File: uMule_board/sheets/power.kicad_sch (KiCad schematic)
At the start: 52 parts, among them Q1 AON6407, U1 TPS62933, U14 TPS62933, U2 TLV761, U3 INA219AxD

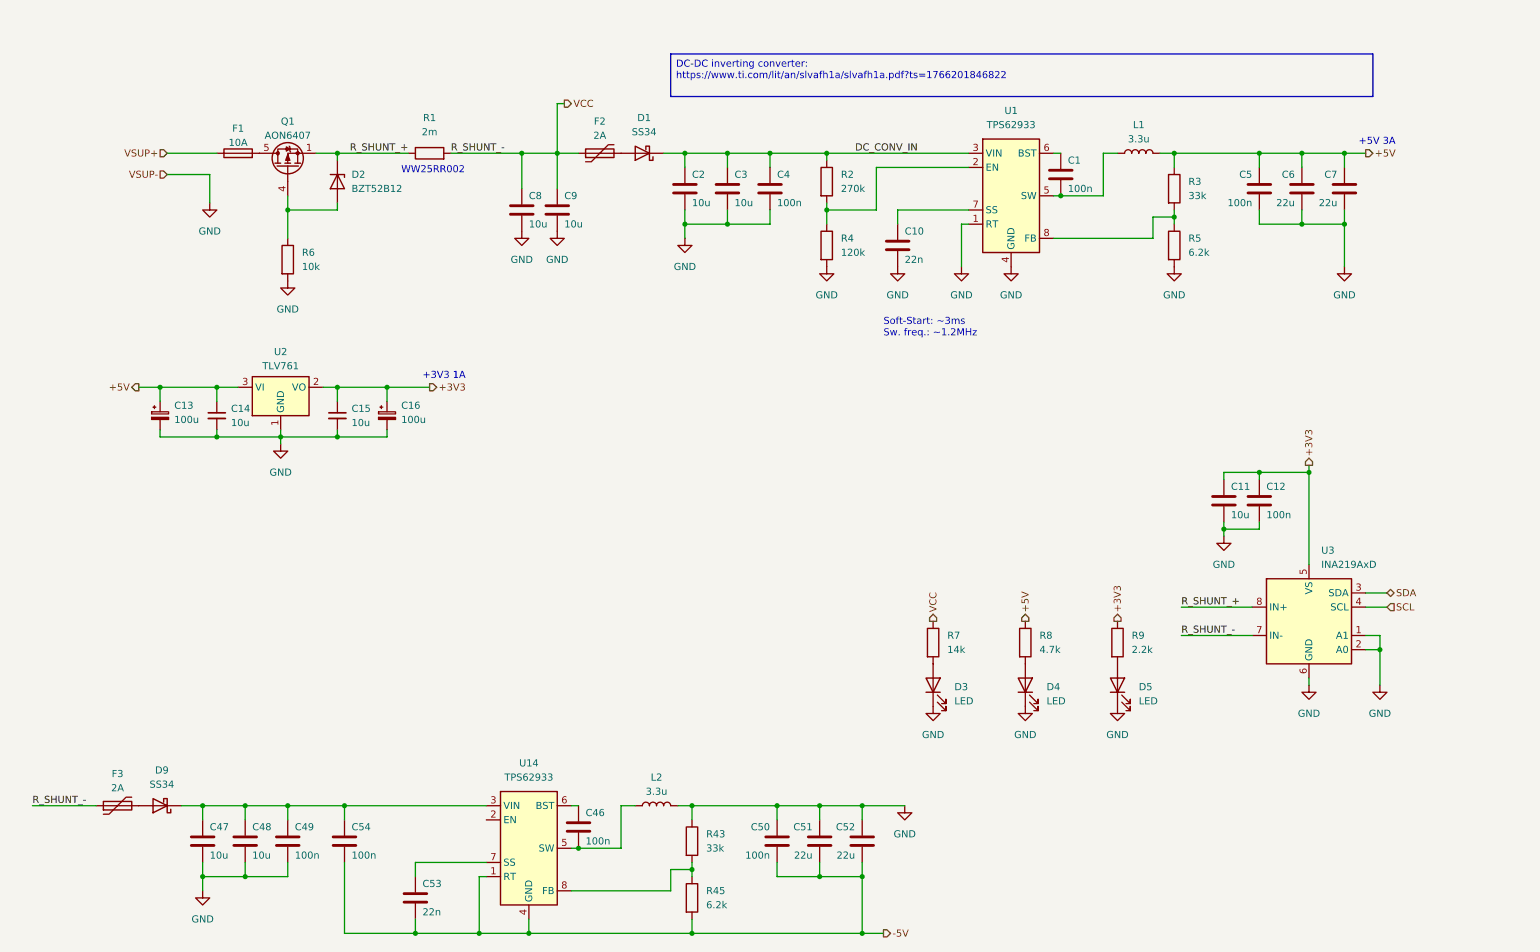
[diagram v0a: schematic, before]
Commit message: sch ready, only missing the pcb
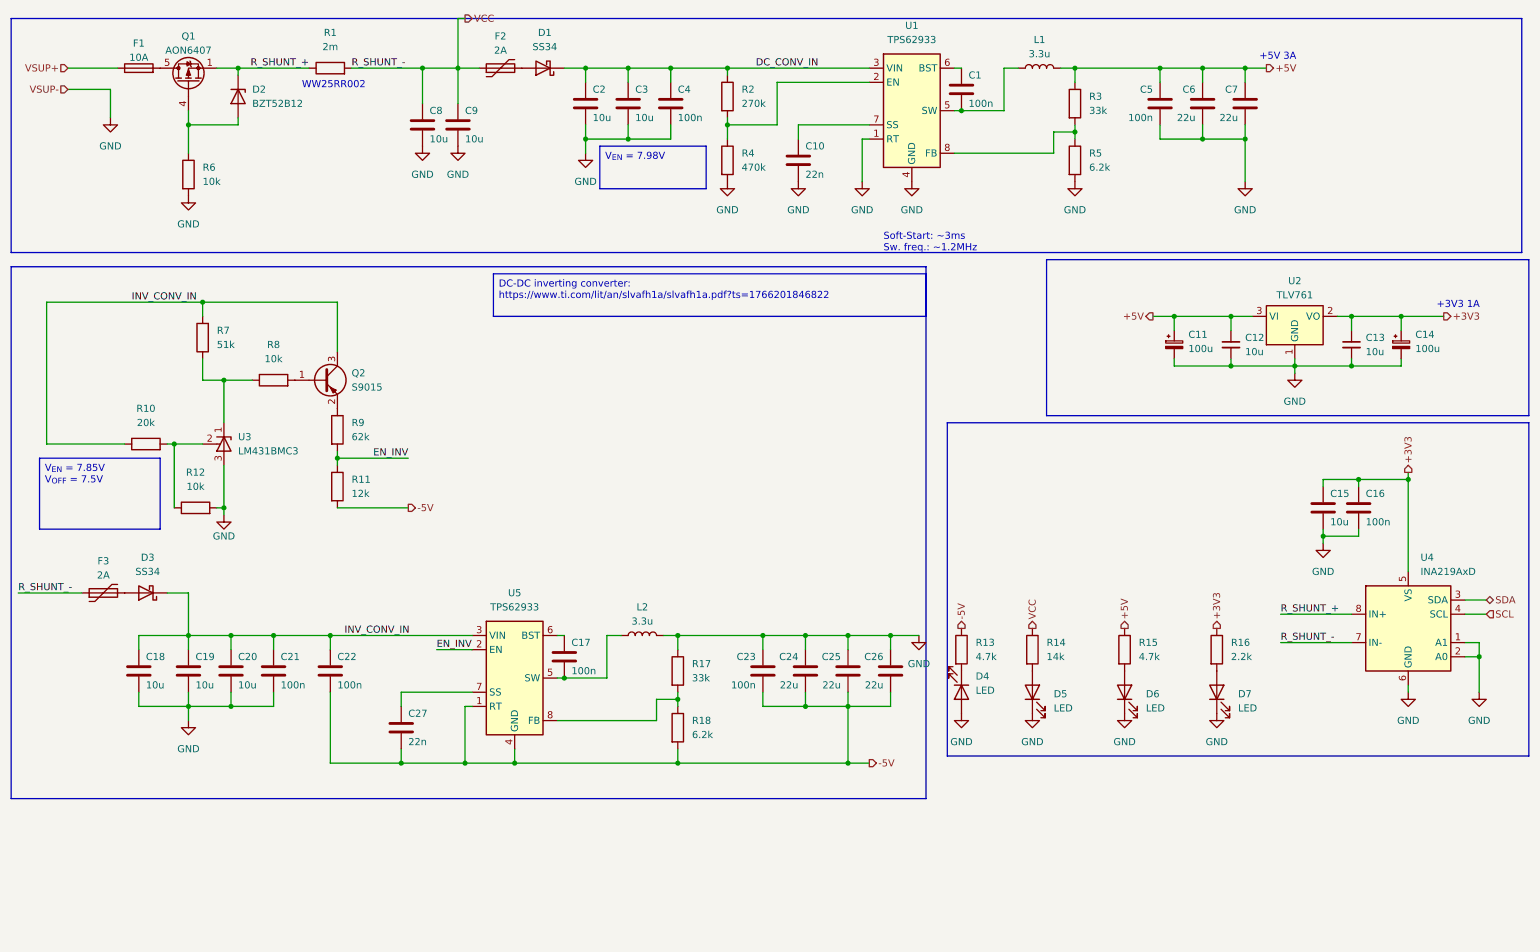
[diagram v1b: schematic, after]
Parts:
- added C18: 10u, Capacitor_SMD:C_0805_2012Metric, symbol Device:C
- added C26: 22u, Capacitor_SMD:C_0805_2012Metric, symbol Device:C
- added D4: LED, LED_SMD:LED_0603_1608Metric_Pad1.05x0.95mm_HandSolder, symbol Device:LED
- added Q2: S9015, Package_TO_SOT_SMD:SOT-23, symbol My_elemets:S9015
- added R10: 20k, Resistor_SMD:R_0603_1608Metric, symbol Device:R
- added R11: 12k, Resistor_SMD:R_0603_1608Metric, symbol Device:R
- added R12, R8: 10k, Resistor_SMD:R_0603_1608Metric, symbol Device:R
- added R13: 4.7k, Resistor_SMD:R_0603_1608Metric, symbol Device:R
- added R7: 51k, Resistor_SMD:R_0603_1608Metric, symbol Device:R
- added R9: 62k, Resistor_SMD:R_0603_1608Metric, symbol Device:R
- added U3: LM431BMC3, Package_TO_SOT_SMD:SOT-23, symbol My_elemets:LM431BMC3
- R4: value 120k -> 470k
- renumbered C13 to C11, C14 to C12, C15 to C13, C16 to C14, C11 to C15, C12 to C16, C46 to C17, C47 to C19, C48 to C20, C49 to C21, C54 to C22, C50 to C23, C51 to C24, C52 to C25, C53 to C27, D9 to D3, D3 to D5, D4 to D6, D5 to D7, R7 to R14, R8 to R15, R9 to R16, R43 to R17, R45 to R18, U3 to U4, U14 to U5
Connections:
- net -5V: now also C26.2, R11.2, R13.1
- net GND: now also C18.2, C26.1, D4.2 (A), R12.2, U3.3 (A)
- net INV_CONV_IN: now reaches C19.1, C20.1, C21.1, C22.1, D3.1 (K), U5.3 (VIN)
- net INV_CONV_IN: now also C18.1, Q2.3 (C), R10.1, R7.2
- net EN_INV: now reaches U5.2 (EN)
- net EN_INV: now also R11.1, R9.2
- new net: R10.2, R12.1, U3.2 (REF)
- new net: R7.1, R8.1, U3.1 (K)
- new net: Q2.1 (B), R8.2
- new net: Q2.2 (E), R9.1
- new net: D4.1 (K), R13.2
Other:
- moved on the sheet: C1, C10, C11, C12, C13, C14, C15, C16, C17, C19, C2, C20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
